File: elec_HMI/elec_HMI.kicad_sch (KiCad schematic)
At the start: 22 parts, among them J1 JST SH, J2 JST SH, U1 PCF8574ATS

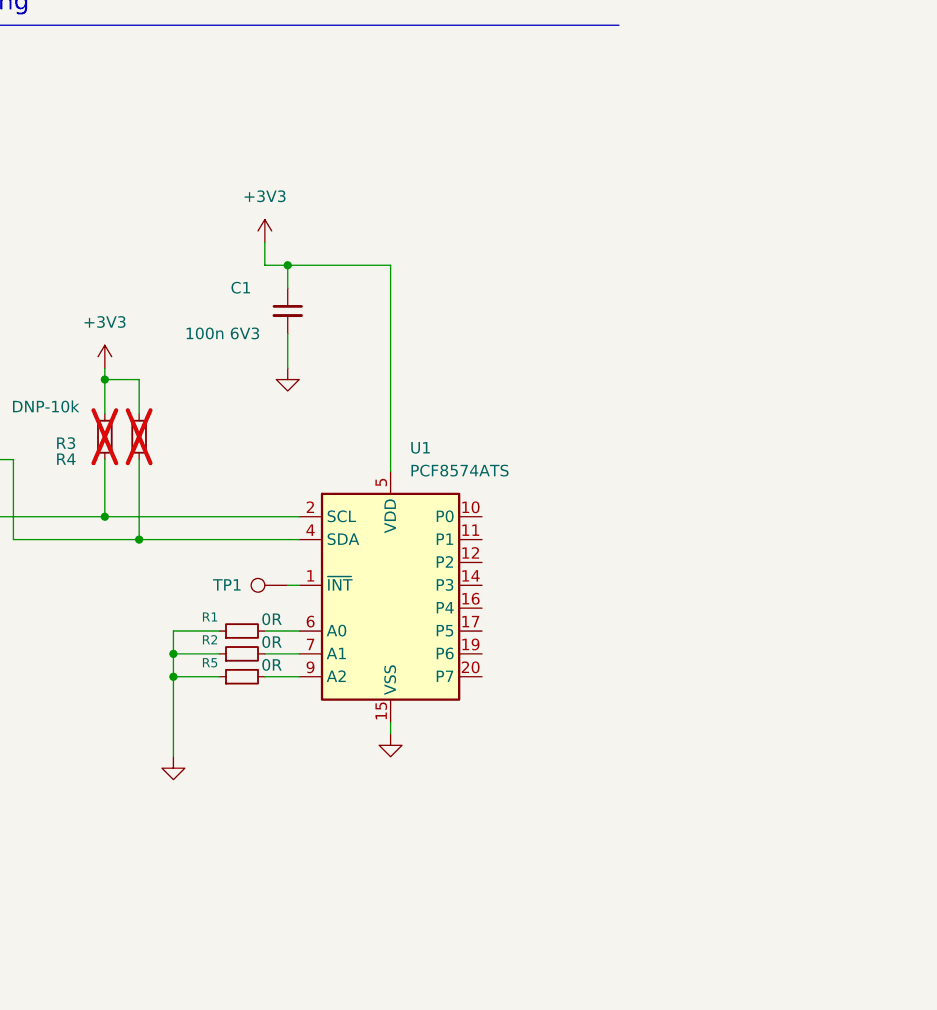
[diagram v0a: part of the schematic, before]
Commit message: [added] Wiring Diagrams
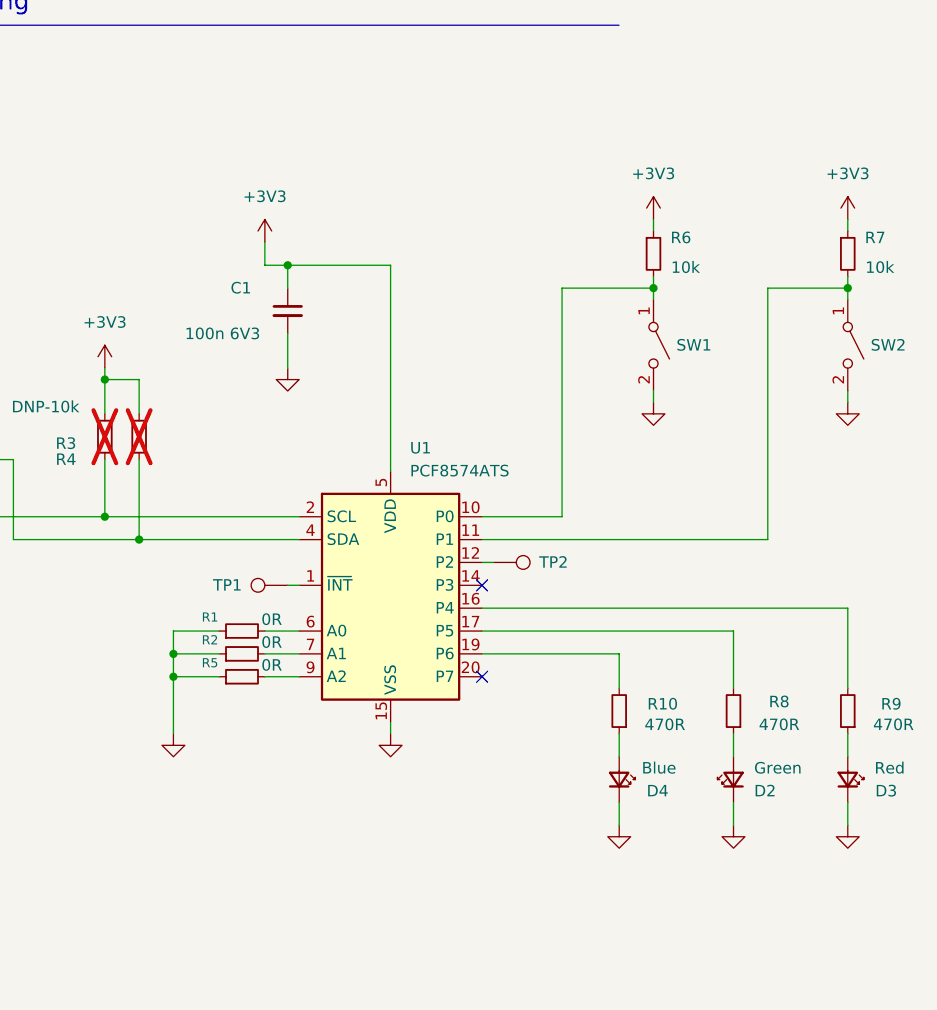
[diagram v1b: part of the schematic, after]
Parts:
- added D2: Green, LED_SMD:LED_0603_1608Metric, symbol Device:LED_Small
- added D3: Red, LED_SMD:LED_0603_1608Metric, symbol Device:LED_Small
- added D4: Blue, LED_SMD:LED_0603_1608Metric, symbol Device:LED_Small
- added R10, R8, R9: 470R, Resistor_SMD:R_0402_1005Metric, symbol Device:R_Small
- added R6, R7: 10k, Resistor_SMD:R_0402_1005Metric, symbol Device:R_Small
- added SW1, SW2: SW_SPST, Button_Switch_Keyboard:SW_Cherry_MX_1.00u_PCB, symbol Switch:SW_SPST
- added TP2: TestPoint, TestPoint:TestPoint_Loop_D2.50mm_Drill1.0mm_LowProfile, symbol Connector:TestPoint
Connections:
- net +3V3: now also R6.1, R7.1
- net GND: now also D2.1 (K), D3.1 (K), D4.1 (K), SW1.2 (B), SW2.2 (B)
- net at U1.10 (P0): now also R6.2, SW1.1 (A)
- net at U1.11 (P1): now also R7.2, SW2.1 (A)
- net at U1.12 (P2): now also TP2.1
- net at U1.16 (P4): now also R9.2
- net at U1.17 (P5): now also R8.2
- net at U1.19 (P6): now also R10.2
- new net: D3.2 (A), R9.1
- new net: D2.2 (A), R8.1
- new net: D4.2 (A), R10.1
- no-connect marks 0 -> 2
